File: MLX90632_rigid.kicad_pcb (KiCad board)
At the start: 2 copper layers, 10 x 10 mm, 5 parts, among them U1 MLX90632SLD-DCB-000-RE

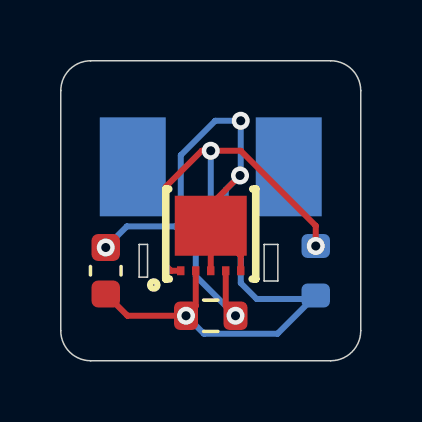
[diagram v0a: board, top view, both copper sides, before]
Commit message: Update for Ver2.0
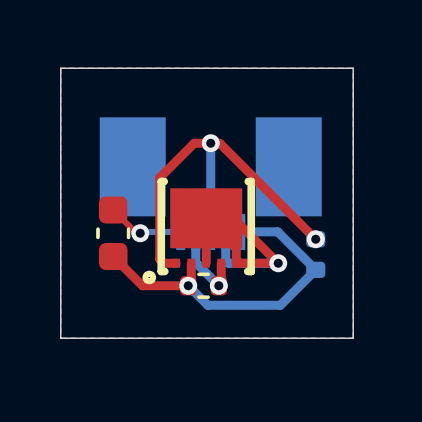
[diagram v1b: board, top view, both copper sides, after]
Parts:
- R1, R2: footprint Resistor_SMD:R_0603_1608Metric -> Resistor_SMD:R_0402_1005Metric
- moved C1 1.27 mm to (158.8, 86.8)
- moved R2 1.03 mm to (161.8, 88.5)
- moved R1 0.54 mm to (165.5, 87.5)
- moved U1 0.29 mm to (161.8, 87.0)
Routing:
- net GND: track 17.3 -> 13.2 mm, vias 3 -> 2
- net +3V3: track 14.2 -> 11.7 mm
- net Net-(U1-SCL): track 4.98 -> 2.90 mm
- added copper zone on B.Cu, net GND
- added copper zone on F.Cu, net GND
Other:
- board size 10 x 10 mm -> 9.8 x 9 mm
